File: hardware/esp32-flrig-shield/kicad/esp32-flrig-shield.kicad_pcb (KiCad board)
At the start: 2 copper layers, 100 x 67 mm, 11 parts, among them J1 RJ45, J2 CYD, J3 S3_HOST, J5 USB-A_B, J6 USB-A_C, J7 ROTOR, U1 ISO7741, U2 AMS1117, U3 PCM5102, U4 INMP441, U5 USB2422

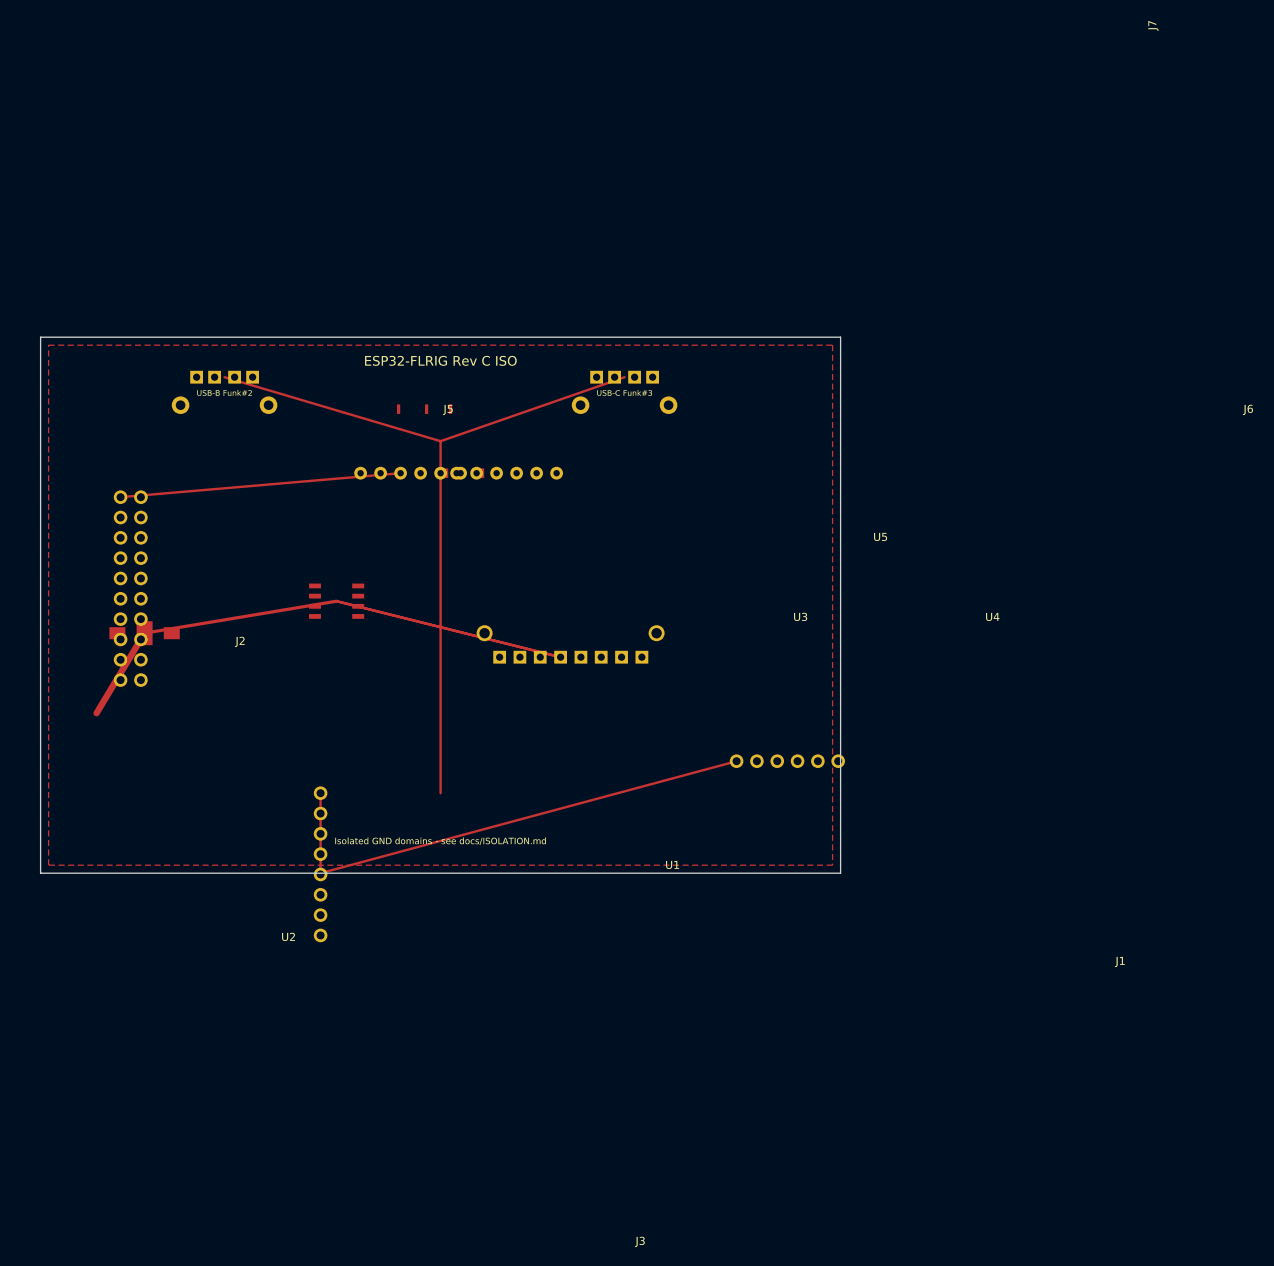
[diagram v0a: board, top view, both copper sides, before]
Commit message: minor correction
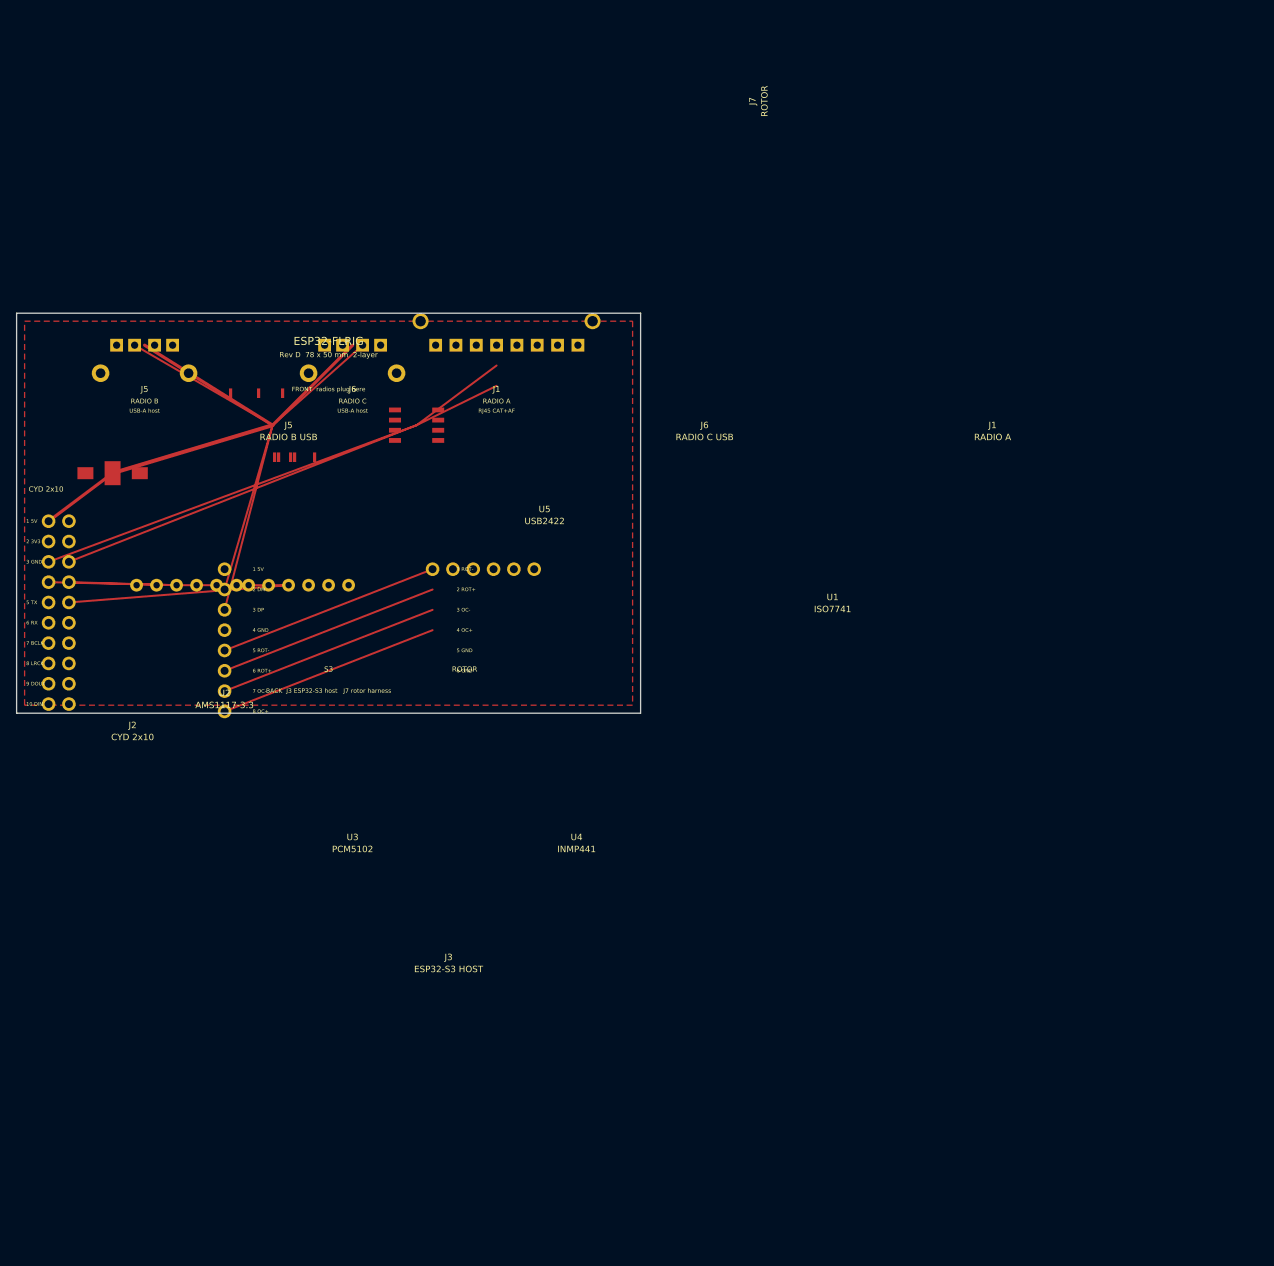
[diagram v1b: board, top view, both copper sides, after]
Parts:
- J1: value RJ45 -> RADIO A
- J2: value CYD -> CYD 2x10
- J3: value S3_HOST -> ESP32-S3 HOST
- J5: value USB-A_B -> RADIO B USB
- J6: value USB-A_C -> RADIO C USB
- U2: value AMS1117 -> AMS1117-3.3
- moved J7 44.9 mm to (54.0, 34.0)
- moved J1 39.8 mm to (62.0, 6.00)
- moved J6 34.2 mm to (44.0, 6.00)
- moved U3 31.3 mm to (22.0, 36.0)
- moved J3 30.5 mm to (28.0, 34.0)
- moved U4 29.5 mm to (36.0, 36.0)
- moved U1 24.2 mm to (52.0, 16.0)
- moved U5 21.1 mm to (34.0, 16.0)
- moved U2 20.4 mm to (14.0, 22.0)
- moved J5 10.8 mm to (18.0, 6.00)
- moved J2 9.49 mm to (6.00, 28.0)
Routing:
- net CAT_ESP_TX: track 0.00 -> 49.1 mm
- net CAT_ESP_RX: track 0.00 -> 46.7 mm
- net ROTOR_BTN_CCW: track 63.9 -> 27.9 mm
- net ROTOR_OC_CW: track 0.00 -> 27.9 mm
- net ROTOR_OC_CCW: track 0.00 -> 27.9 mm
- net ROTOR_BTN_CW: track 0.00 -> 27.9 mm
- net +5V_BUS: track 36.0 -> 63.9 mm
- net I2S_DIN: track 0.00 -> 27.5 mm
- net USB_OTG_DM: track 0.00 -> 21.4 mm
- net USB_OTG_DP: track 44.0 -> 23.8 mm
- net I2S_BCLK: track 35.1 -> 16.0 mm
- net CAT_RX_RADIO: track 28.9 -> 11.1 mm
- net CAT_TX_RADIO: track 28.9 -> 12.5 mm
- net I2S_DOUT: track 0.00 -> 14.0 mm
- net I2S_LRCK: track 0.00 -> 13.5 mm
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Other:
- board size 100 x 67 mm -> 78 x 50 mm
- board text added: "1 5V"
- board text added: "1 ROT-"
- board text added: "10 DIN"
- board text added: "2 3V3"
- board text added: "2 DM"
- board text added: "2 ROT+"
- board text added: "3 DP"
- board text added: "3 GND"
- board text added: "3 OC-"
- board text added: "4 GND"
- board text added: "4 OC+"
- board text added: "5 GND"
- board text added: "5 ROT-"
- board text added: "5 TX"
- board text added: "6 GND"
- board text added: "6 ROT+"
- board text added: "6 RX"
- board text added: "7 BCLK"
- board text added: "7 OC-"
- board text added: "8 LRCK"
- board text added: "8 OC+"
- board text added: "9 DOUT"
- board text added: "BACK J3 ESP32-S3 host J7 rotor harness"
- board text added: "CYD 2x10"
- board text added: "ESP32-FLRIG"
- board text added: "FRONT radios plug here"
- board text added: "J1"
- board text added: "J5"
- board text added: "J6"
- board text added: "RADIO A"
- board text added: "RADIO B"
- board text added: "RADIO C"
- board text added: "RJ45 CAT+AF"
- board text added: "ROTOR"
- board text added: "Rev D 78 x 50 mm 2-layer"
- board text added: "S3"
- board text added: "USB-A host"
- board text removed: "ESP32-FLRIG Rev C ISO"
- board text removed: "Isolated GND domains - see docs/ISOLATION.md"
- board text removed: "USB-B Funk#2"
- board text removed: "USB-C Funk#3"
